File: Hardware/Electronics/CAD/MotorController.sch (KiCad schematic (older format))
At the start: 14 parts, among them J1 MPE 094-1-006, J2 CONN_01X03, J3 Screw_Terminal_1x02, J5 CONN_01X04, SW2 SW_DPST_x2, U1 LD1117S33CTR, U2 MAX471, U3 TMC2130, U4 ESP-12E, U5 HiLink, U6 Nema

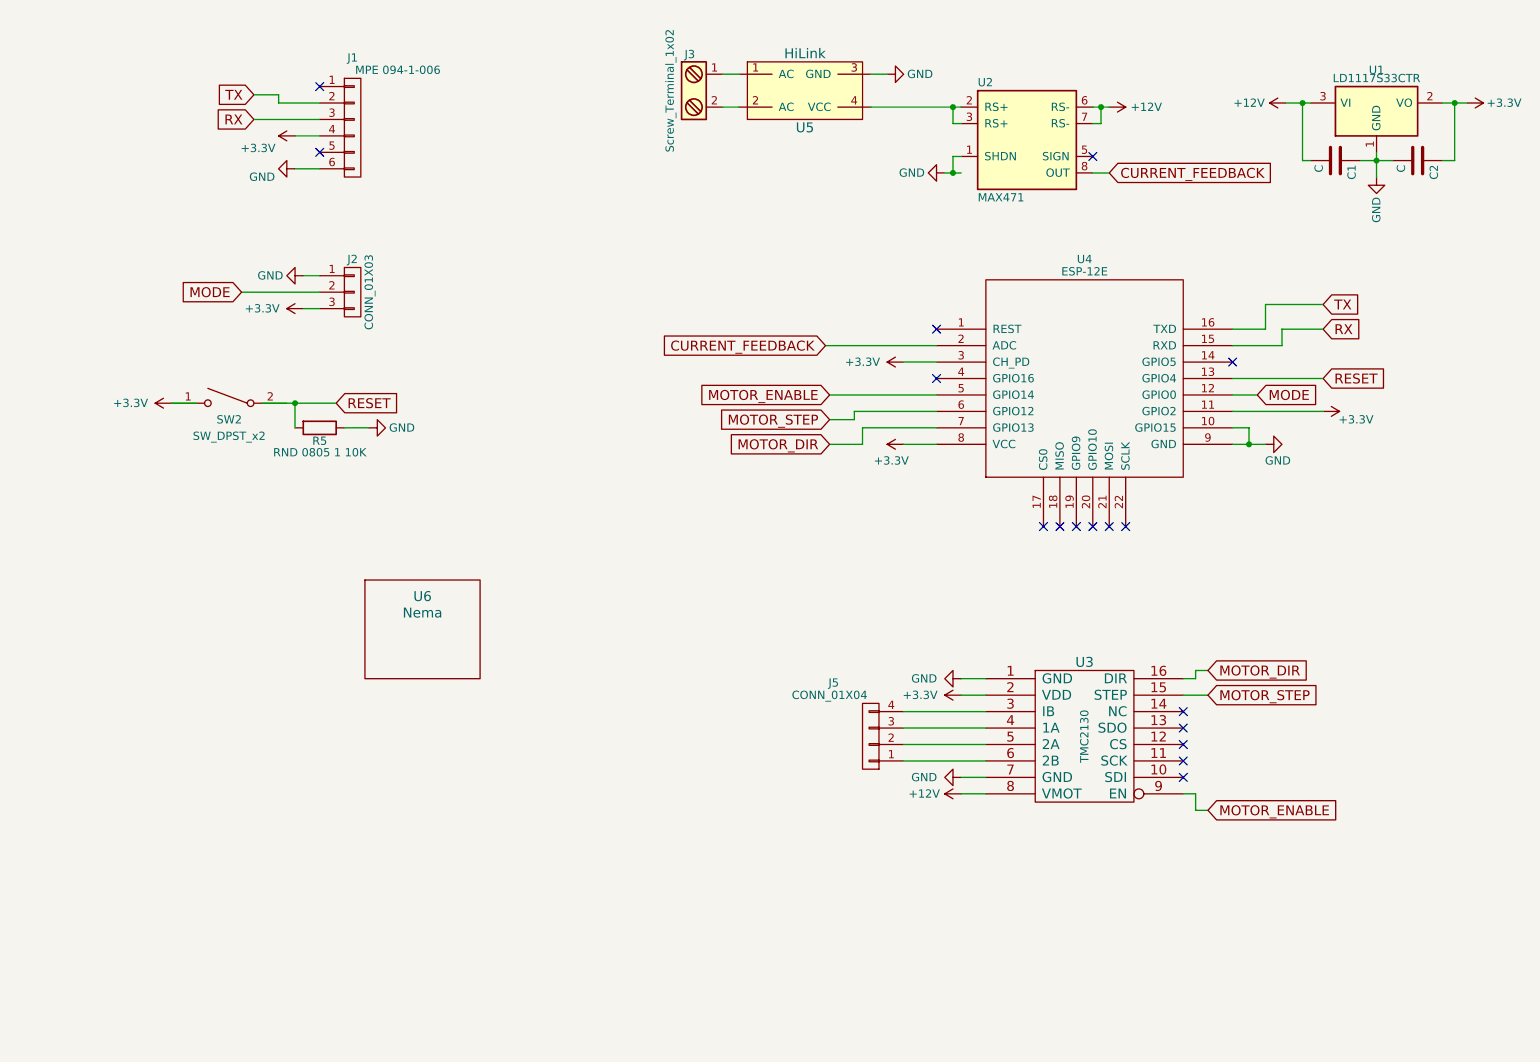
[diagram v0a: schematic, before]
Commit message: revision1.0.0 for electrical hardware
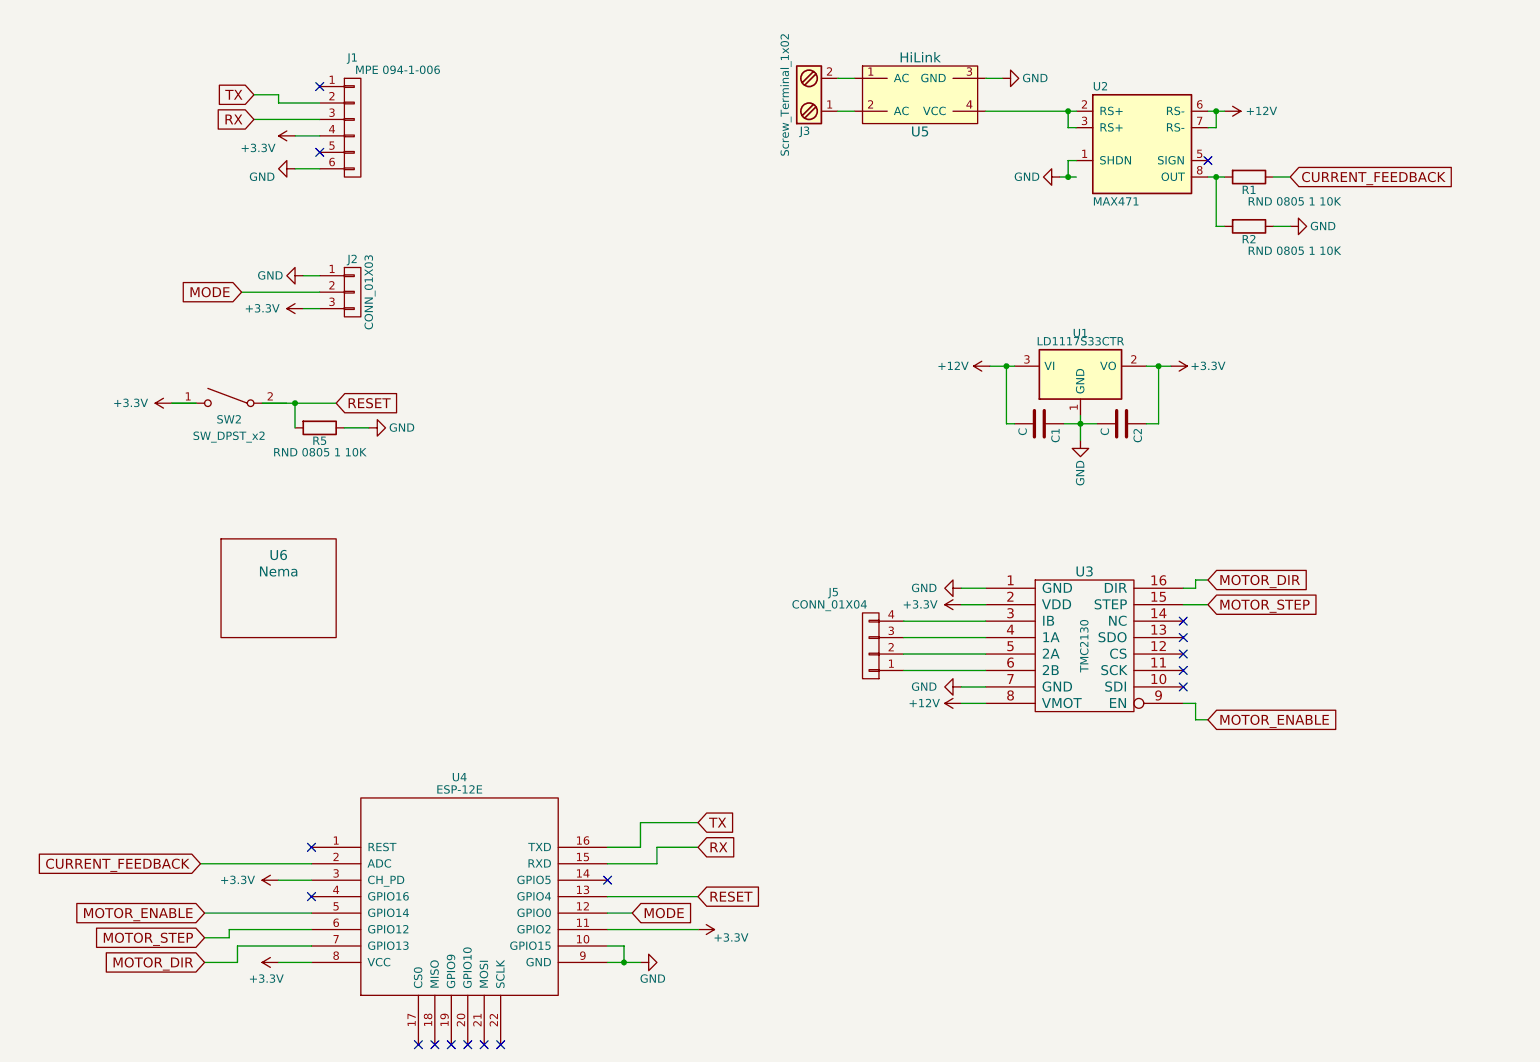
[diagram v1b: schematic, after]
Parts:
- added R1, R2: RND 0805 1 10K, Resistors_SMD:R_0805, symbol R
- J1: footprint Socket_Strips:Socket_Strip_Angled_1x06_Pitch2.54mm -> Pin_Headers:Pin_Header_Straight_1x06_Pitch2.54mm_SMD_Pin1Right
- J2: footprint Pin_Headers:Pin_Header_Angled_1x03_Pitch2.54mm -> Pin_Headers:Pin_Header_Straight_1x03_Pitch2.54mm_SMD_Pin1Right
- J3: footprint WAGO:WAGO_2pin -> Terminal:SolderTerminal
- J5: footprint Pin_Headers:Pin_Header_Angled_1x04_Pitch2.54mm -> Terminal:Pin_Header_SMD_Angled_2.54mm
- U5: footprint HiLink:HiLink -> HiLink:HLK-PM01
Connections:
- net CURRENT_FEEDBACK: now also R1.1; no longer U2.8 (OUT)
- net GND: now also R2.1
- net at U5.1 (AC): now also J3.2; no longer J3.1
- net at U5.2 (AC): now also J3.1; no longer J3.2
- new net: R1.2, R2.2, U2.8 (OUT)
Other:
- moved on the sheet: C1, C2, J3, J5, U1, U2, U3, U4, U5, U6
